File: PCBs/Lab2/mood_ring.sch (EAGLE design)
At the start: 8 parts

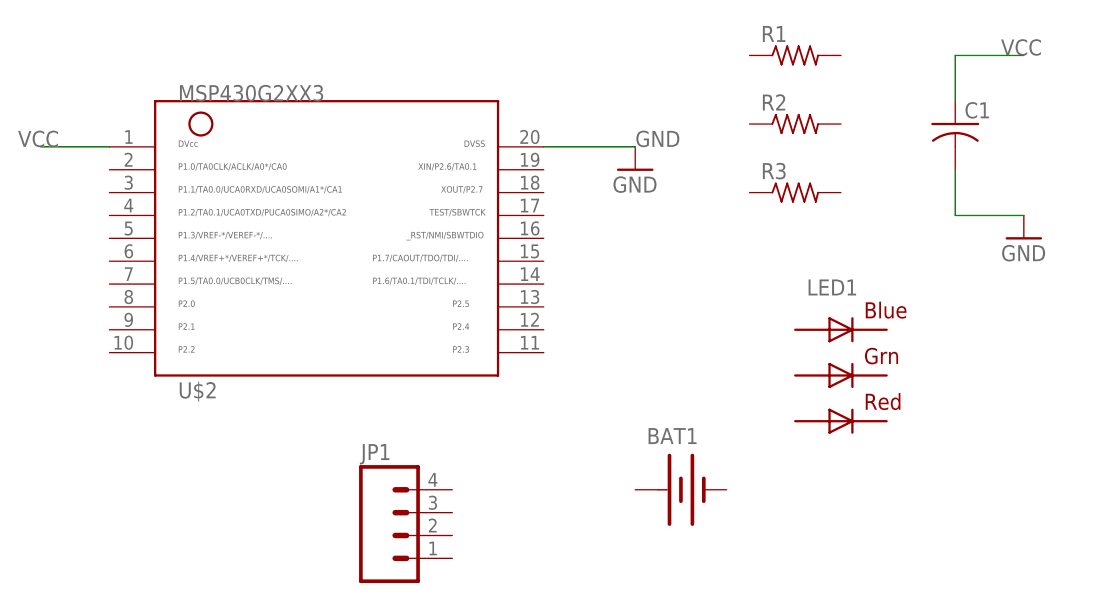
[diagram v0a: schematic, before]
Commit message: added lab 2
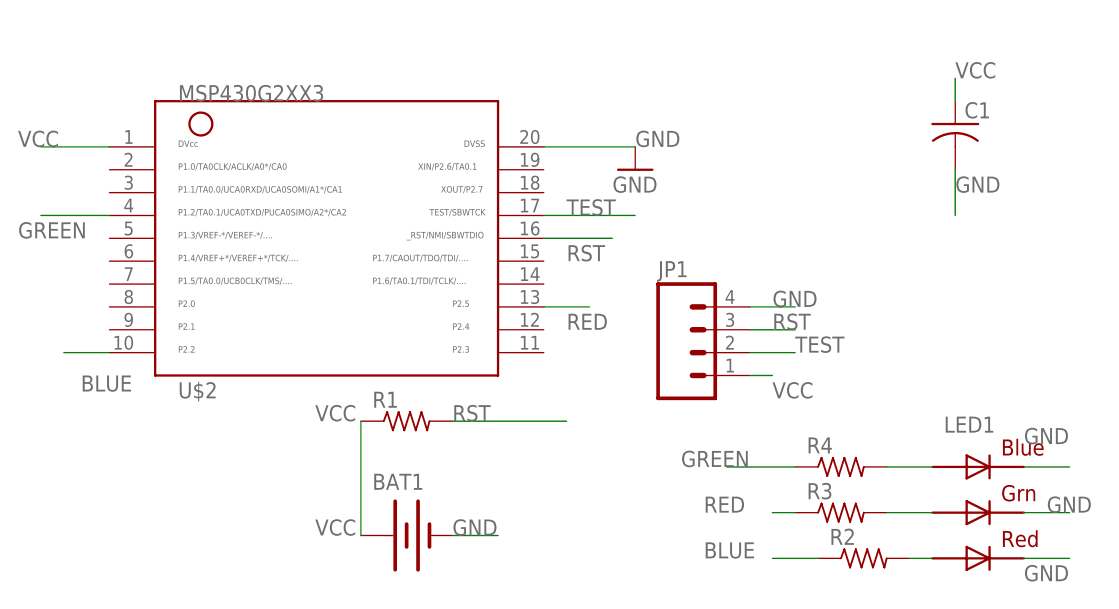
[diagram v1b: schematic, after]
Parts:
- added R4: (no value), resistor:R-US_R1206
- U$2: value MSP430G2XX3PDIP -> MSP430G2XX3TSSOP; device ELEC327:MSP430G2XX3PDIP -> ELEC327:MSP430G2XX3TSSOP
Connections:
- new net BLUE: R2.1, U$2.10
- new net GREEN: R4.1, U$2.4
- new net N$1: LED1.BLUE_A, R4.2
- new net N$2: LED1.GREEN_A, R3.2
- new net N$3: LED1.RED_A, R2.2
- new net RED: R3.1, U$2.13
- new net RST: JP1.3, R1.2, U$2.16
- new net TEST: JP1.2, U$2.17
- net GND: now also BAT1.-, JP1.4, LED1.BLUE_C, LED1.GREEN_C, LED1.RED_C
- net VCC: now also BAT1.+, JP1.1, R1.1
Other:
- moved on the sheet: BAT1, JP1, LED1, R1, R2, R3
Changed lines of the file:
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@@
 <?xml version="1.0" encoding="utf-8"?>
 <!DOCTYPE eagle SYSTEM "eagle.dtd">
-<eagle version="6.5.0">
+<eagle version="7.2.0">
 <drawing>
 <settings>
@@
 <setting verticaltext="up"/>
 </settings>
-<grid distance="0.1" unitdist="inch" unit="inch" style="lines" multiple="1" display="yes" altdistance="0.01" altunitdist="inch" altunit="inch"/>
+<grid distance="0.1" unitdist="inch" unit="inch" style="lines" multiple="1" display="no" altdistance="0.01" altunitdist="inch" altunit="inch"/>
 <layers>
 <layer number="1" name="Top" color="4" fill="1" visible="no" active="no"/>
@@
 </classes>
 <parts>
-<part name="U$2" library="ELEC327" deviceset="MSP430G2XX3" device="PDIP"/>
+<part name="U$2" library="ELEC327" deviceset="MSP430G2XX3" device="TSSOP" value="MSP430G2XX3TSSOP"/>
 <part name="JP1" library="SparkFun" deviceset="M04" device="LOCK"/>
 <part name="R1" library="resistor" deviceset="R-US_" device="R1206"/>
@@
 <part name="C1" library="resistor" deviceset="C-US" device="C1206"/>
 <part name="GND1" library="supply1" deviceset="GND" device=""/>
-<part name="GND2" library="supply1" deviceset="GND" device=""/>
+<part name="R4" library="resistor" deviceset="R-US_" device="R1206"/>
 </parts>
 <sheets>
@@
 <instances>
 <instance part="U$2" gate="G$1" x="-22.86" y="172.72"/>
-<instance part="JP1" gate="G$1" x="-15.24" y="137.16"/>
-<instance part="R1" gate="G$1" x="27.94" y="190.5"/>
-<instance part="R2" gate="G$1" x="27.94" y="182.88"/>
-<instance part="R3" gate="G$1" x="27.94" y="175.26"/>
-<instance part="LED1" gate="G$1" x="33.02" y="154.94"/>
-<instance part="BAT1" gate="G$1" x="15.24" y="142.24"/>
+<instance part="JP1" gate="G$1" x="17.78" y="157.48"/>
+<instance part="R1" gate="G$1" x="-15.24" y="149.86"/>
+<instance part="R2" gate="G$1" x="35.56" y="134.62"/>
+<instance part="R3" gate="G$1" x="33.02" y="139.7"/>
+<instance part="LED1" gate="G$1" x="48.26" y="139.7"/>
+<instance part="BAT1" gate="G$1" x="-15.24" y="137.16"/>
 <instance part="C1" gate="G$1" x="45.72" y="182.88"/>
 <instance part="GND1" gate="1" x="10.16" y="177.8"/>
-<instance part="GND2" gate="1" x="53.34" y="170.18"/>
+<instance part="R4" gate="G$1" x="33.02" y="144.78"/>
 </instances>
 <busses>
@@
 <net name="VCC" class="0">
 <segment>
+<pinref part="BAT1" gate="G$1" pin="+"/>
+<pinref part="R1" gate="G$1" pin="1"/>
+<wire x1="-20.32" y1="137.16" x2="-20.32" y2="149.86" width="0.1524" layer="91"/>
+<label x="-25.4" y="149.86" size="1.778" layer="95"/>
+<label x="-25.4" y="137.16" size="1.778" layer="95"/>
+</segment>
+<segment>
 <pinref part="U$2" gate="G$1" pin="1"/>
 <wire x1="-48.26" y1="180.34" x2="-55.88" y2="180.34" width="0.1524" layer="91"/>
@@
 </segment>
 <segment>
+<pinref part="JP1" gate="G$1" pin="1"/>
+<wire x1="22.86" y1="154.94" x2="25.4" y2="154.94" width="0.1524" layer="91"/>
+<label x="25.4" y="152.4" size="1.778" layer="95"/>
+</segment>
+<segment>
 <pinref part="C1" gate="G$1" pin="1"/>
-<wire x1="45.72" y1="185.42" x2="45.72" y2="190.5" width="0.1524" layer="91"/>
-<wire x1="45.72" y1="190.5" x2="53.34" y2="190.5" width="0.1524" layer="91"/>
-<label x="50.8" y="190.5" size="1.778" layer="95"/>
+<wire x1="45.72" y1="185.42" x2="45.72" y2="187.96" width="0.1524" layer="91"/>
+<label x="45.72" y="187.96" size="1.778" layer="95"/>
 </segment>
 </net>
 <net name="GND" class="0">
 <segment>
+<pinref part="GND1" gate="1" pin="GND"/>
 <pinref part="U$2" gate="G$1" pin="20"/>
 <wire x1="0" y1="180.34" x2="10.16" y2="180.34" width="0.1524" layer="91"/>
 <label x="10.16" y="180.34" size="1.778" layer="95"/>
-<pinref part="GND1" gate="1" pin="GND"/>
+</segment>
+<segment>
+<pinref part="LED1" gate="G$1" pin="BLUE_C"/>
+<wire x1="53.34" y1="144.78" x2="58.42" y2="144.78" width="0.1524" layer="91"/>
+<label x="53.34" y="147.32" size="1.778" layer="95"/>
+</segment>
+<segment>
+<pinref part="LED1" gate="G$1" pin="RED_C"/>
+<wire x1="53.34" y1="134.62" x2="58.42" y2="134.62" width="0.1524" layer="91"/>
+<label x="53.34" y="132.08" size="1.778" layer="95"/>
+</segment>
+<segment>
+<pinref part="BAT1" gate="G$1" pin="-"/>
+<wire x1="-10.16" y1="137.16" x2="-5.08" y2="137.16" width="0.1524" layer="91"/>
+<label x="-10.16" y="137.16" size="1.778" layer="95"/>
+</segment>
+<segment>
+<pinref part="JP1" gate="G$1" pin="4"/>
+<wire x1="22.86" y1="162.56" x2="27.94" y2="162.56" width="0.1524" layer="91"/>
+<label x="25.4" y="162.56" size="1.778" layer="95"/>
 </segment>
 <segment>
 <pinref part="C1" gate="G$1" pin="2"/>
 <wire x1="45.72" y1="177.8" x2="45.72" y2="172.72" width="0.1524" layer="91"/>
-<wire x1="45.72" y1="172.72" x2="53.34" y2="172.72" width="0.1524" layer="91"/>
-<pinref part="GND2" gate="1" pin="GND"/>
-</segment>
-</net>
+<label x="45.72" y="175.26" size="1.778" layer="95"/>
+</segment>
+<segment>
+<pinref part="LED1" gate="G$1" pin="GREEN_C"/>
+<wire x1="53.34" y1="139.7" x2="58.42" y2="139.7" width="0.1524" layer="91"/>
+<label x="55.88" y="139.7" size="1.778" layer="95"/>
+</segment>
+</net>
+<net name="RST" class="0">
+<segment>
+<pinref part="R1" gate="G$1" pin="2"/>
+<wire x1="-10.16" y1="149.86" x2="2.54" y2="149.86" width="0.1524" layer="91"/>
+<label x="-10.16" y="149.86" size="1.778" layer="95"/>
+</segment>
+<segment>
+<wire x1="0" y1="170.18" x2="7.62" y2="170.18" width="0.1524" layer="91"/>
+<pinref part="U$2" gate="G$1" pin="16"/>
+<label x="2.54" y="167.64" size="1.778" layer="95"/>
+</segment>
+<segment>
+<pinref part="JP1" gate="G$1" pin="3"/>
+<wire x1="22.86" y1="160.02" x2="27.94" y2="160.02" width="0.1524" layer="91"/>
+<label x="25.4" y="160.02" size="1.778" layer="95"/>
+</segment>
+</net>
+<net name="TEST" class="0">
+<segment>
+<pinref part="U$2" gate="G$1" pin="17"/>
+<wire x1="0" y1="172.72" x2="10.16" y2="172.72" width="0.1524" layer="91"/>
+<label x="2.54" y="172.72" size="1.778" layer="95"/>
+</segment>
+<segment>
+<pinref part="JP1" gate="G$1" pin="2"/>
+<wire x1="22.86" y1="157.48" x2="27.94" y2="157.48" width="0.1524" layer="91"/>
+<label x="27.94" y="157.48" size="1.778" layer="95"/>
+</segment>
+</net>
+<net name="RED" class="0">
+<segment>
+<pinref part="U$2" gate="G$1" pin="13"/>
+<wire x1="0" y1="162.56" x2="5.08" y2="162.56" width="0.1524" layer="91"/>
+<label x="2.54" y="160.02" size="1.778" layer="95"/>
+</segment>
+<segment>
+<pinref part="R3" gate="G$1" pin="1"/>
+<wire x1="25.4" y1="139.7" x2="27.94" y2="139.7" width="0.1524" layer="91"/>
+<label x="17.78" y="139.7" size="1.778" layer="95"/>
+</segment>
+</net>
+<net name="BLUE" class="0">
+<segment>
+<pinref part="U$2" gate="G$1" pin="10"/>
+<wire x1="-48.26" y1="157.48" x2="-53.34" y2="157.48" width="0.1524" layer="91"/>
+<label x="-45.72" y="154.94" size="1.778" layer="95" rot="R180"/>
+</segment>
+<segment>
+<pinref part="R2" gate="G$1" pin="1"/>
+<wire x1="30.48" y1="134.62" x2="25.4" y2="134.62" width="0.1524" layer="91"/>
+<label x="17.78" y="134.62" size="1.778" layer="95"/>
+</segment>
+</net>
+<net name="GREEN" class="0">
+<segment>
+<pinref part="U$2" gate="G$1" pin="4"/>
+<wire x1="-48.26" y1="172.72" x2="-55.88" y2="172.72" width="0.1524" layer="91"/>
+<label x="-58.42" y="170.18" size="1.778" layer="95"/>
+</segment>
+<segment>
+<pinref part="R4" gate="G$1" pin="1"/>
+<wire x1="27.94" y1="144.78" x2="20.32" y2="144.78" width="0.1524" layer="91"/>
+<label x="15.24" y="144.78" size="1.778" layer="95"/>
+</segment>
+</net>
+<net name="N$1" class="0">
+<segment>
+<pinref part="R4" gate="G$1" pin="2"/>
+<pinref part="LED1" gate="G$1" pin="BLUE_A"/>
+<wire x1="38.1" y1="144.78" x2="43.18" y2="144.78" width="0.1524" layer="91"/>
+</segment>
+</net>
+<net name="N$2" class="0">
+<segment>
+<pinref part="R3" gate="G$1" pin="2"/>
+<pinref part="LED1" gate="G$1" pin="GREEN_A"/>
+<wire x1="38.1" y1="139.7" x2="43.18" y2="139.7" width="0.1524" layer="91"/>
+</segment>
+</net>
+<net name="N$3" class="0">
+<segment>
+<pinref part="LED1" gate="G$1" pin="RED_A"/>
+<pinref part="R2" gate="G$1" pin="2"/>
+<wire x1="43.18" y1="134.62" x2="40.64" y2="134.62" width="0.1524" layer="91"/>
+</segment>
+</net>
